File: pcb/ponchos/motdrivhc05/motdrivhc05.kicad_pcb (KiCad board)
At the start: 2 copper layers, 53.3 x 64.1 mm, 21 parts, among them J1 Screw_Terminal_1x06, J3 GW-040, J4 CONN_01X02, Q1 TIP31, U1 L293

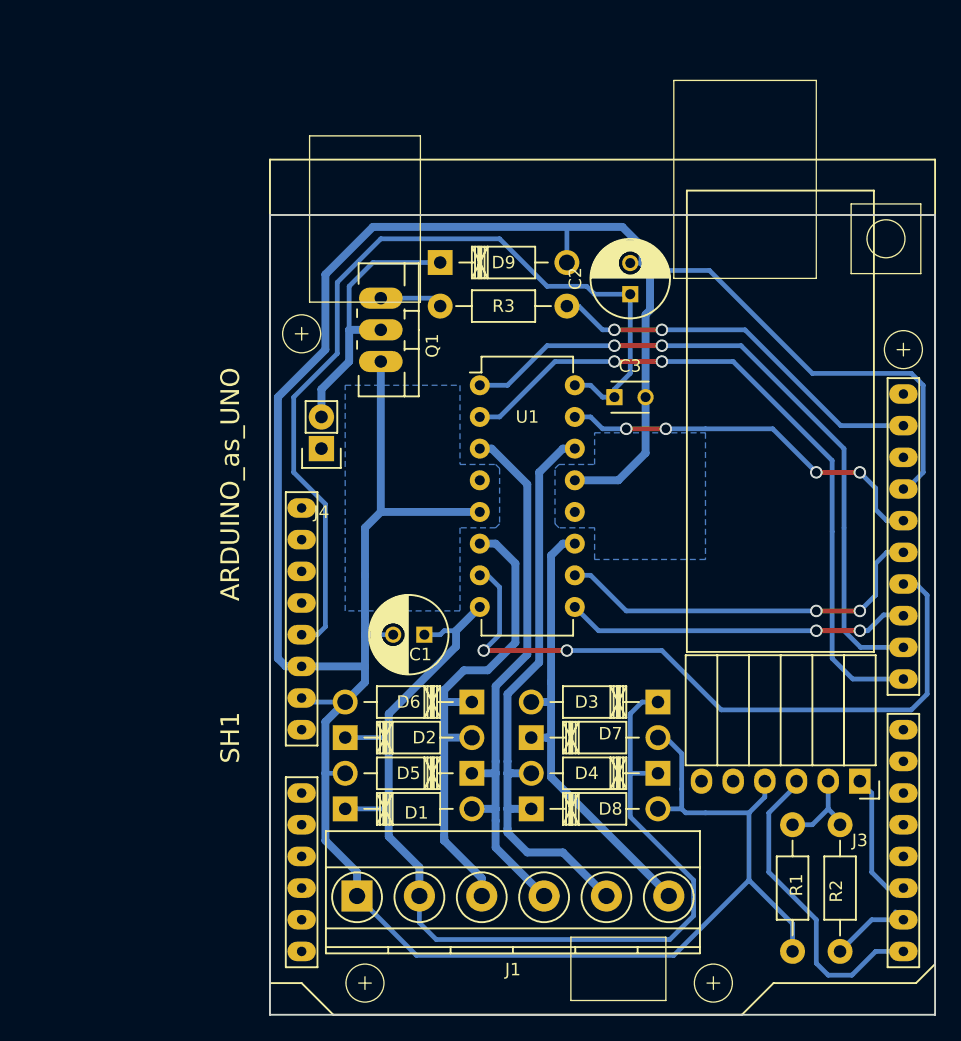
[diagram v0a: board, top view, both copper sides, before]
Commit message: Primer versión de PCB terminada.
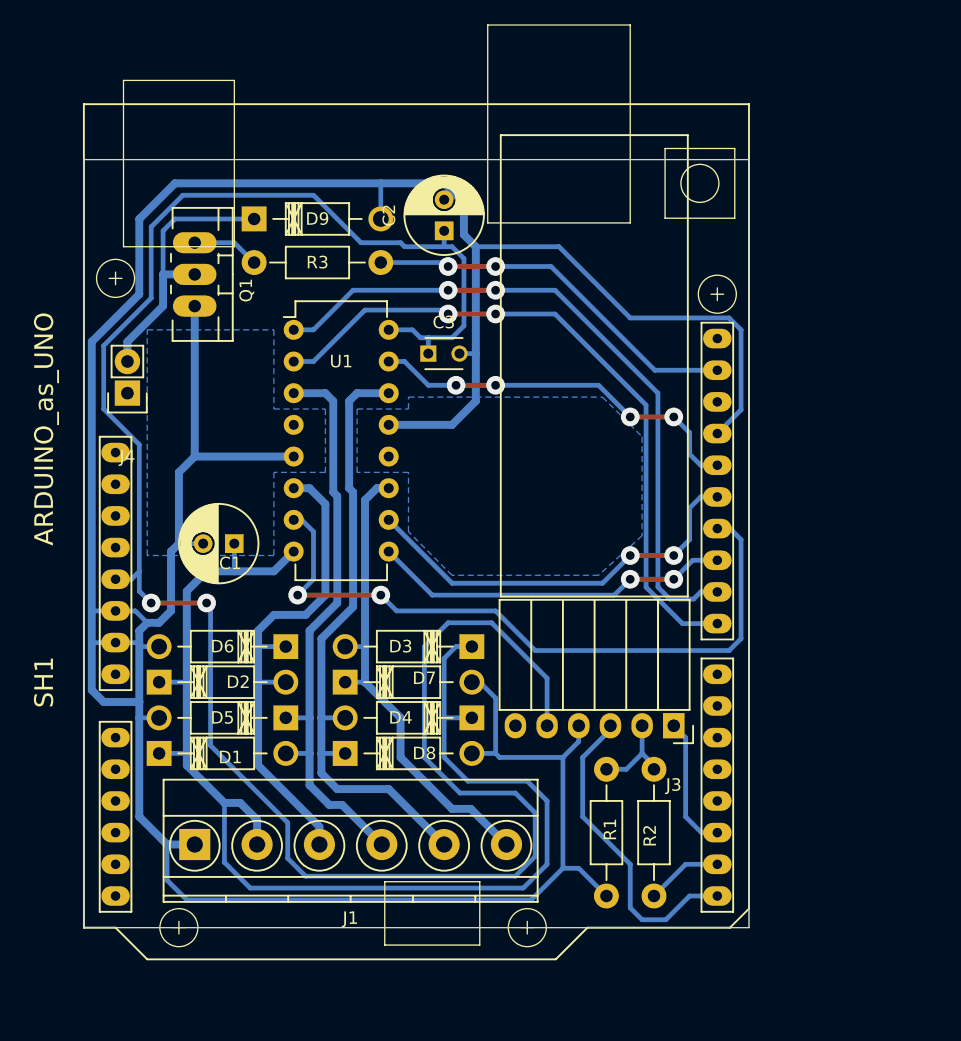
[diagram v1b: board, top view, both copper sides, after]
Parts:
- moved C1 16.9 mm to (44.1, 63.2)
- moved J4 16.2 mm to (35.6, 51.1)
- moved C2 15.8 mm to (61.0, 38.1)
- moved D3 15.6 mm to (63.2, 71.4)
- moved D4 15.6 mm to (63.2, 77.2)
- moved J3 15.6 mm to (79.4, 77.8)
- moved R1 15.6 mm to (77.8, 91.4)
- moved D1 15.6 mm to (38.1, 80.0)
- moved D2 15.6 mm to (38.1, 74.3)
- moved D5 15.6 mm to (48.3, 77.2)
- moved D6 15.6 mm to (48.3, 71.4)
- moved Q1 15.6 mm to (41.0, 41.6)
- moved R2 15.6 mm to (74.0, 81.3)
- moved SH1 15.6 mm to (58.7, 62.2)
- moved U1 15.6 mm to (48.9, 46.0)
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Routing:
- net +5V: track 71.4 -> 166.5 mm, vias 0 -> 2
- net VCC: track 86.3 -> 100.5 mm
- net GND: track 257.6 -> 270.8 mm
- net Net-(D1-Pad2): track 44.6 -> 46.9 mm
- net /M3A: track 31.0 -> 32.8 mm
- net Net-(D4-Pad2): track 48.7 -> 50.5 mm
- net /ME34: track 27.7 -> 29.0 mm
- net /ME12: track 53.9 -> 54.9 mm
- net /M1A: track 55.7 -> 54.7 mm
- net /BT_RXD: track 7.03 -> 6.13 mm
- net Net-(D3-Pad2): track 38.0 -> 38.7 mm
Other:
- board size 53.3 x 64.1 mm -> 53.3 x 61.6 mm
